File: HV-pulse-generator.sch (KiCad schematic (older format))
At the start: 13 parts, among them J1 CONN_01X03, J2 Pin1=TTL Pin2=GND, J3 Pin1=24V Pin2=GND, J4 CONN_01X02, J5 Pin1=TTL Pin2=GND, Q2 FQP3P50, Q5 FQP13N50

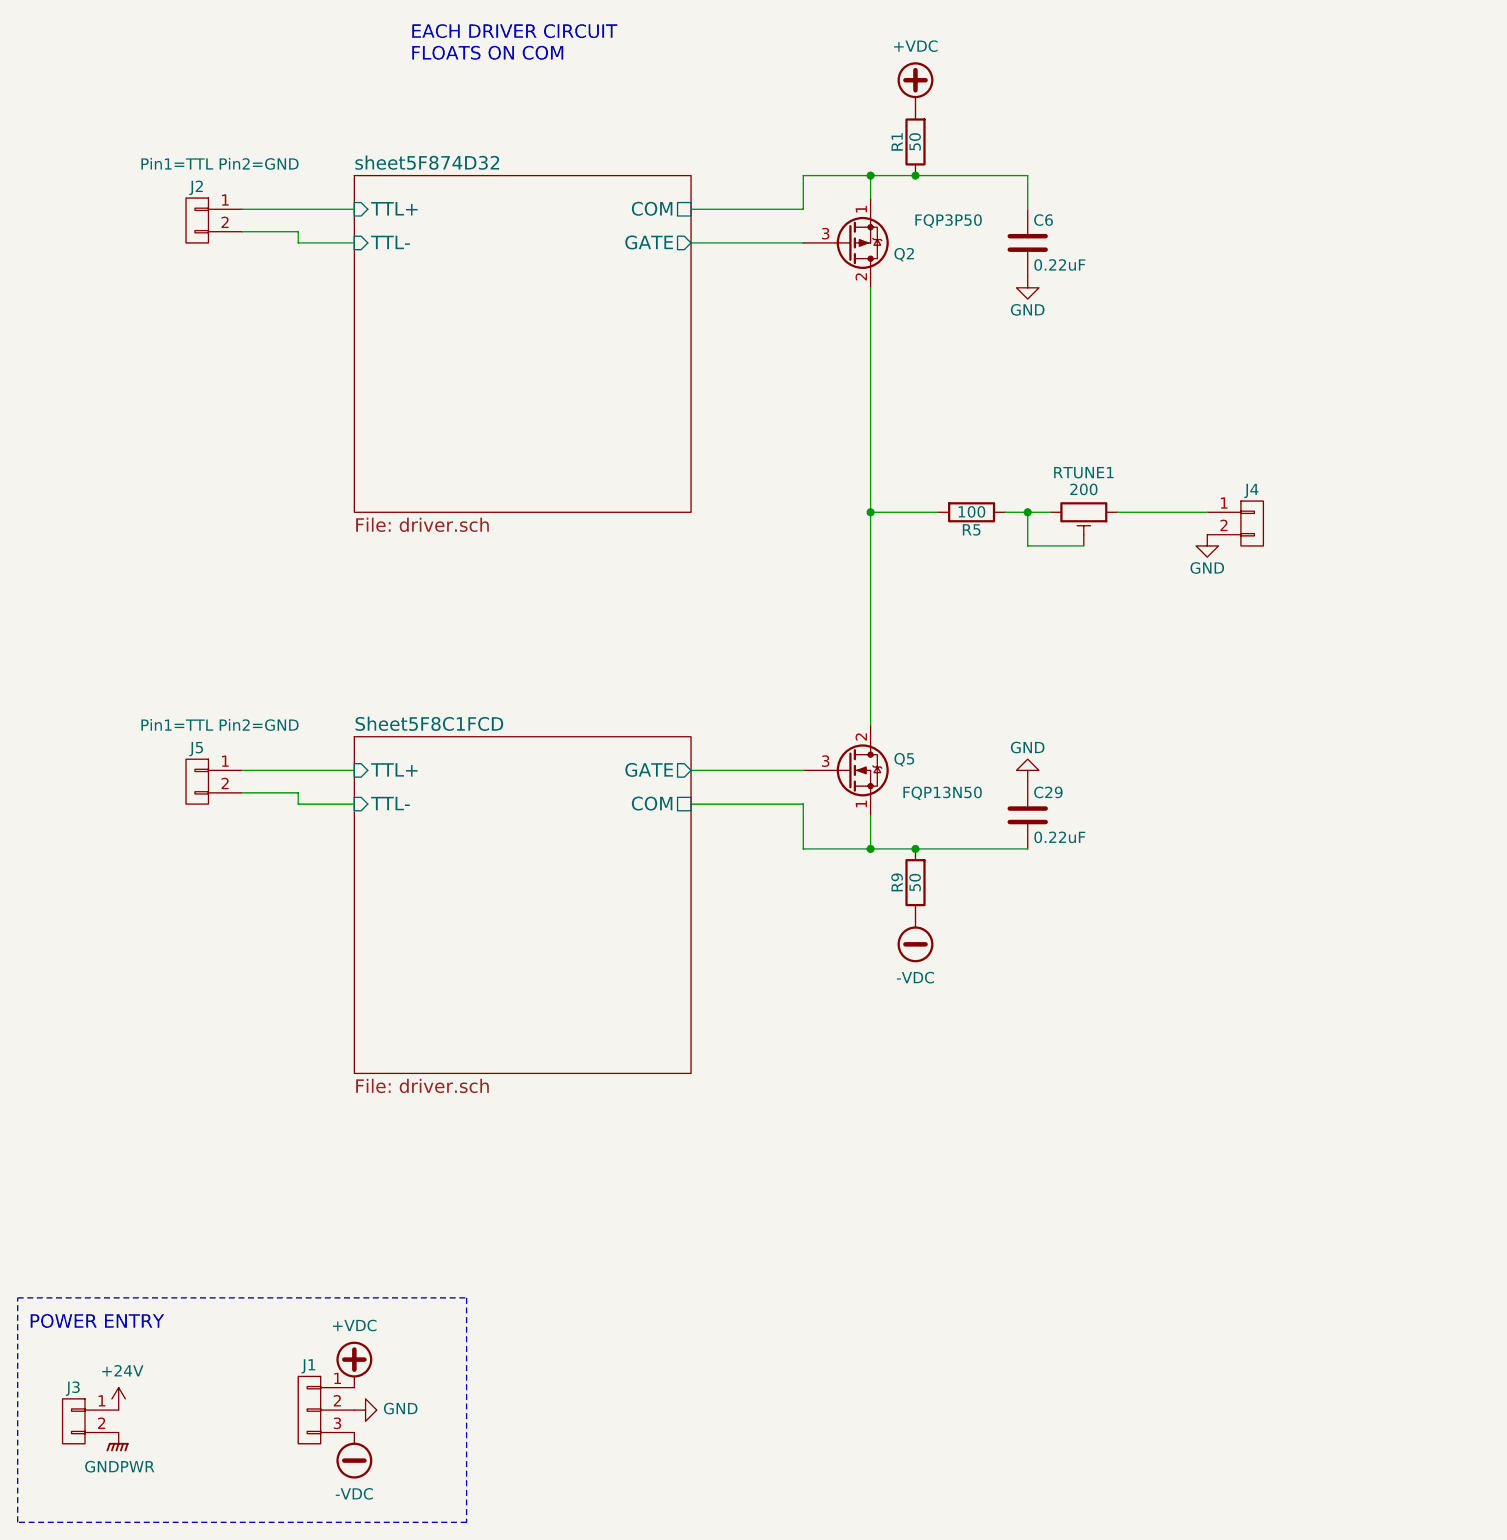
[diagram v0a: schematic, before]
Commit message: 2.0.0
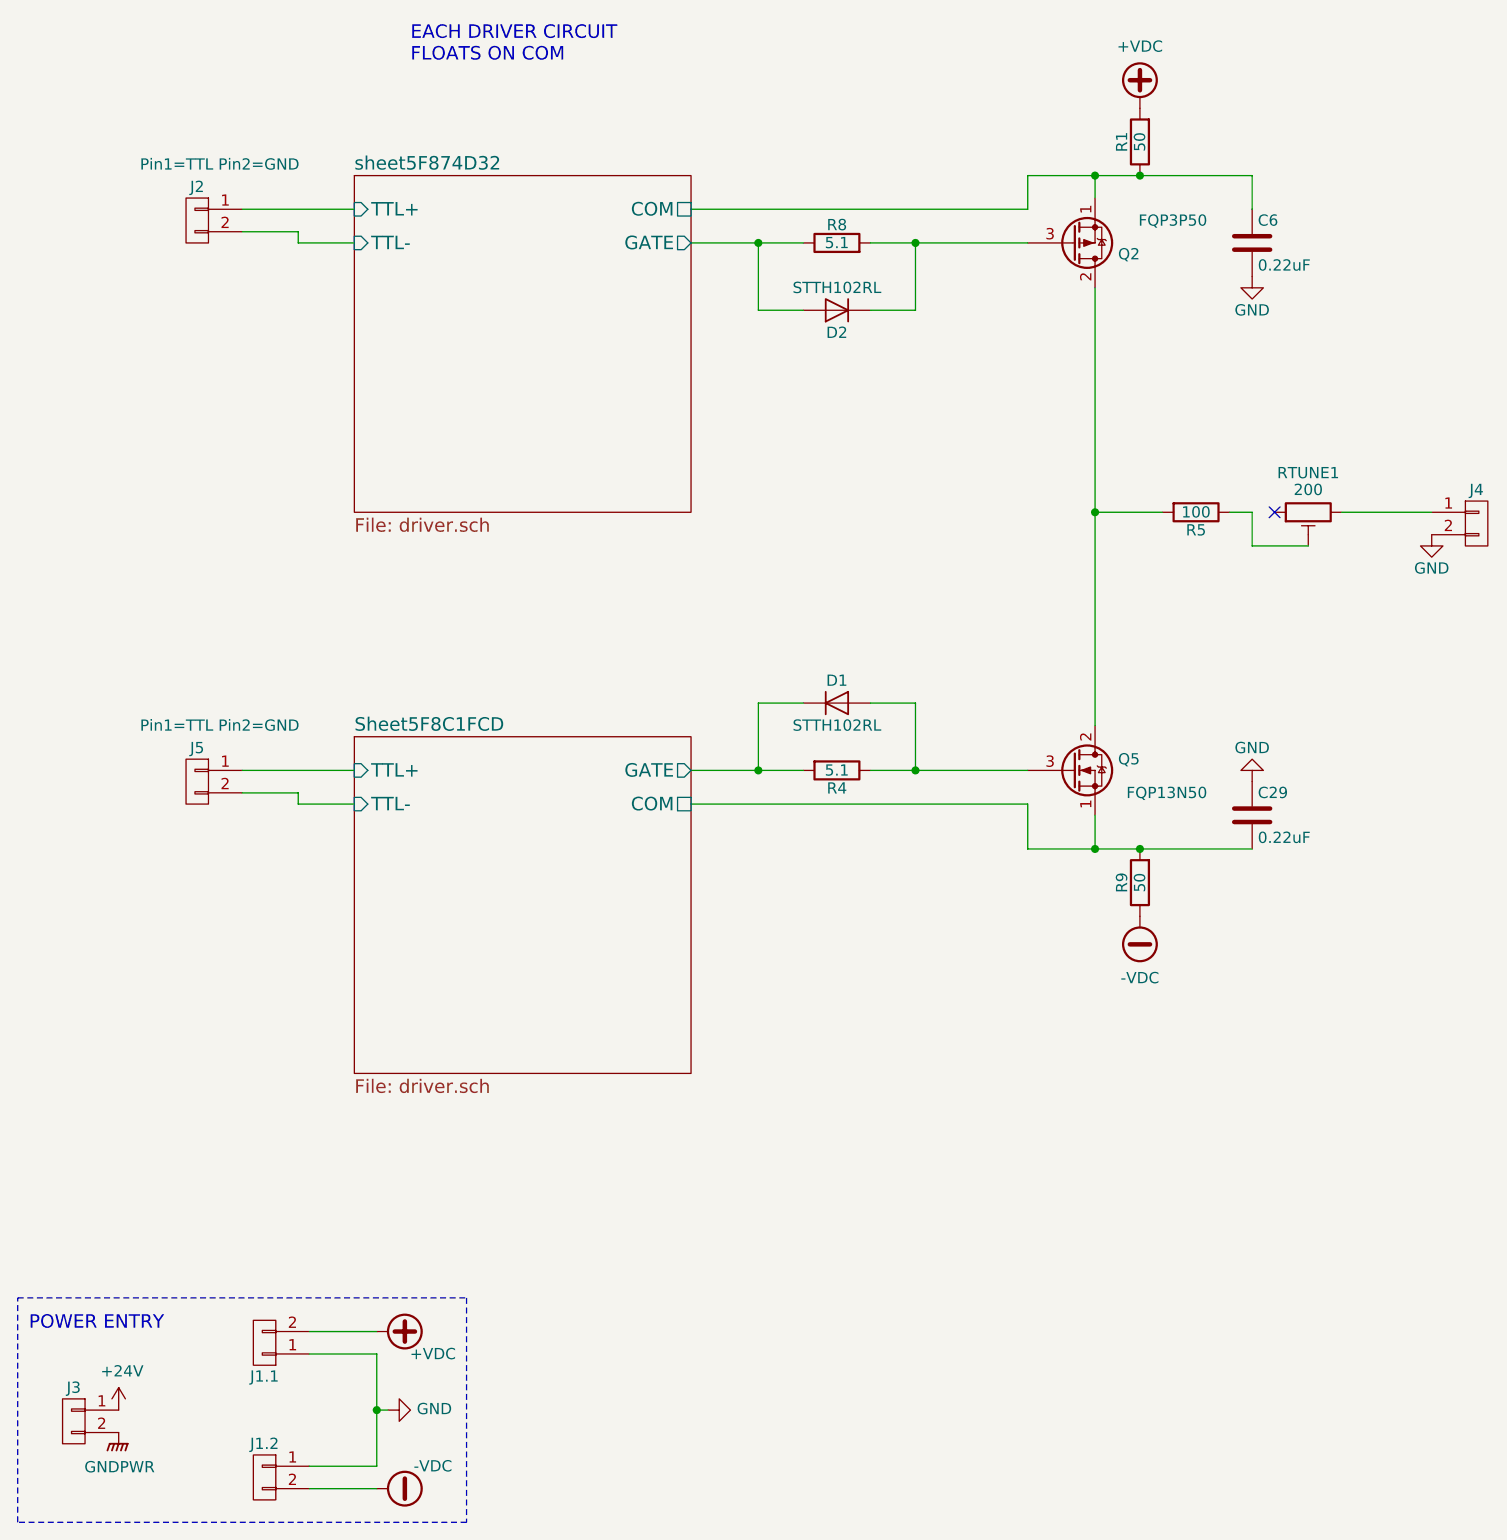
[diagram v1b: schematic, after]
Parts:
- removed J1: CONN_01X03, hvhf:Pin_Header_Molex_10-32-1031, symbol HV-pulse-generator-rescue:CONN_01X03
- added D1, D2: STTH102RL, hvhf:Diode_DO-41_SOD81_Horizontal_RM10, symbol HV-pulse-generator-rescue:D
- added J1.1, J1.2: Pin1=24V Pin2=GND, Connector_PinHeader_2.54mm:PinHeader_1x02_P2.54mm_Vertical, symbol HV-pulse-generator-rescue:CONN_01X02
- added R4, R8: 5.1, hvhf:Resistor_Horizontal_RM15mm, symbol HV-pulse-generator-rescue:R
- J4: footprint hvhf:Pin_Header_Molex_10-32-1021 -> Connector_PinHeader_2.54mm:PinHeader_1x02_P2.54mm_Vertical
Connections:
- net +VDC: now also J1.1.2 (P2)
- net -VDC: now also J1.2.2 (P2)
- net GND: now also J1.1.1 (P1), J1.2.1 (P1)
- net Sheet5F8C1FCD/GATE: now also D1.1 (K), R4.2; no longer Q5.3 (G)
- net sheet5F874D32/GATE: now also D2.2 (A), R8.1; no longer Q2.3 (G)
- net at R5.1, RTUNE1.2: no longer RTUNE1.3
- net at J4.1 (P1): now also RTUNE1.3; no longer RTUNE1.1
- new net: D2.1 (K), Q2.3 (G), R8.2
- new net: D1.2 (A), Q5.3 (G), R4.1
- no-connect marks 0 -> 1
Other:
- moved on the sheet: C29, C6, J4, Q2, Q5, R1, R5, R9, RTUNE1
